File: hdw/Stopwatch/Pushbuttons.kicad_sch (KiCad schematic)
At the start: 41 parts, among them SW701 Cap_Touch, SW702 Cap_Touch, SW703 Cap_Touch, U701 AT42QT1010-TSHR, U702 TLV71330PDBV, U703 TLV71330PDBV, U704 74LVC1G80, U705 74LVC1G17, U706 TLV71330PDBV, U707 AT42QT1010-TSHR, U708 AT42QT1010-TSHR, U709 74LVC1G17, U710 74LVC1G17

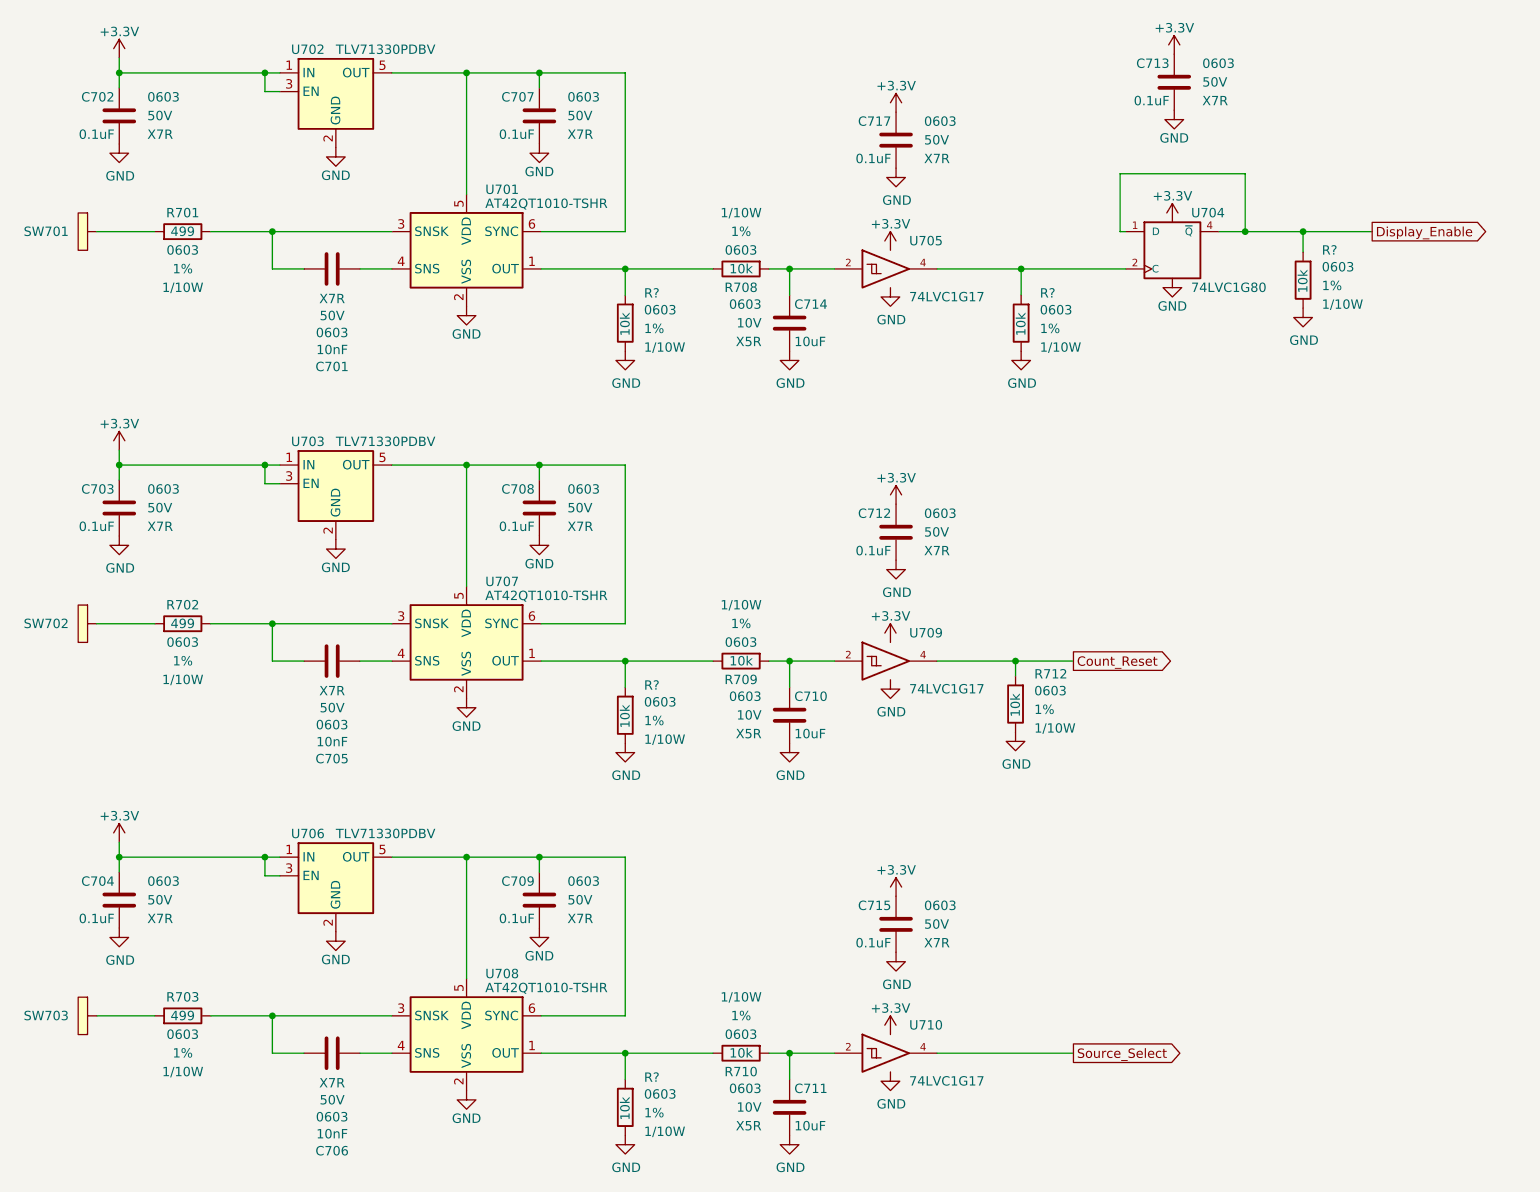
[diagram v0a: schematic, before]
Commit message: started sch work
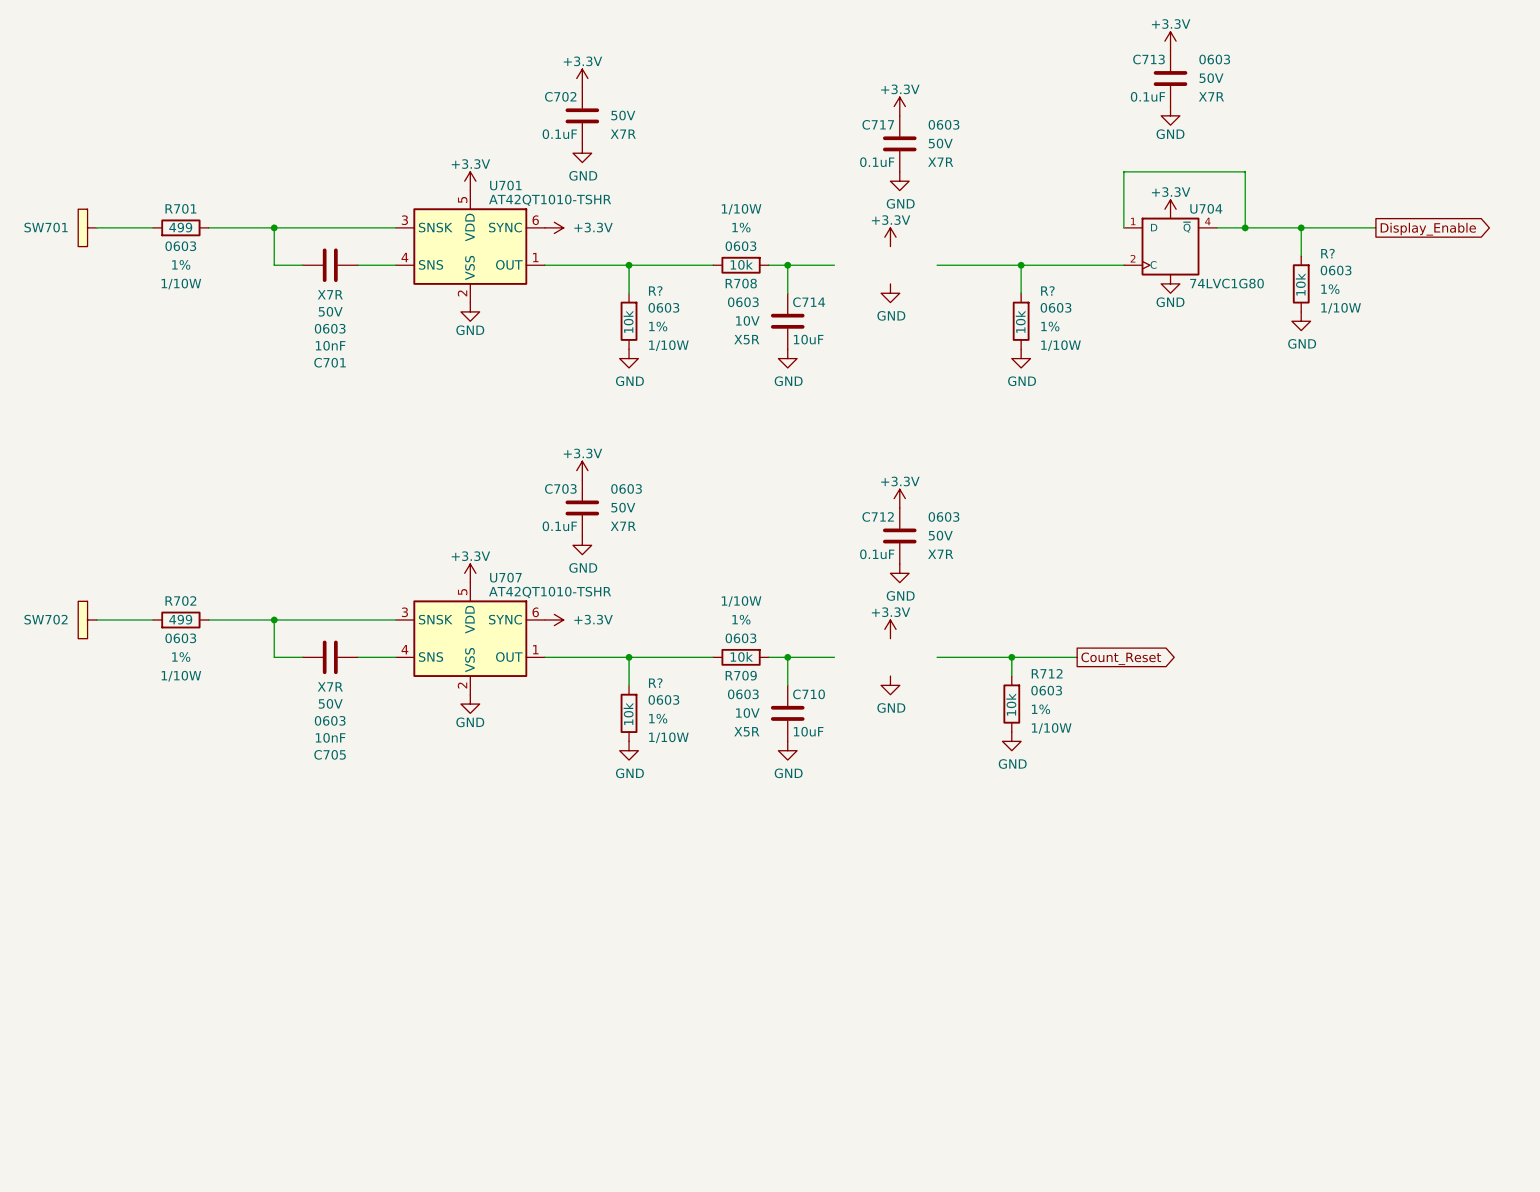
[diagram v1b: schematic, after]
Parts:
- removed C704, C707, C708, C709, C715: 0.1uF, Capacitors_SMD:C_0603, symbol Custom_Library:C_Custom
- removed C706: 10nF, Capacitors_SMD:C_0603, symbol Custom_Library:C_Custom
- removed C711: 10uF, Capacitors_SMD:C_0603, symbol Custom_Library:C_Custom
- removed R703: 499, Resistors_SMD:R_0603, symbol Custom_Library:R_Custom
- removed R710, R?: 10k, Resistors_SMD:R_0603, symbol Custom_Library:R_Custom
- removed SW703: Cap_Touch, Custom Footprints Library:Capacitive_Touch_Pad, symbol Custom_Library:Cap_Touch
- removed U702, U703, U706: TLV71330PDBV, Package_TO_SOT_SMD:SOT-23-5, symbol Incrementor-rescue:TLV71330PDBV-Regulator_Linear
- removed U705, U709, U710: 74LVC1G17, TO_SOT_Packages_SMD:SOT-353_SC-70-5, symbol Custom_Library:74LVC1G17_Power
- removed U708: AT42QT1010-TSHR, TO_SOT_Packages_SMD:SOT-23-6, symbol Sensor_Touch:AT42QT1010-TSHR
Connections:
- net +3V3: now also U701.5 (VDD), U701.6 (SYNC), U707.5 (VDD), U707.6 (SYNC)
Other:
- moved on the sheet: C701, C702, C703, C705, C712, C713, C717, R701, R702, R708, R709, R712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
